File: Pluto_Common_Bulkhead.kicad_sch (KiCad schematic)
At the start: 52 parts

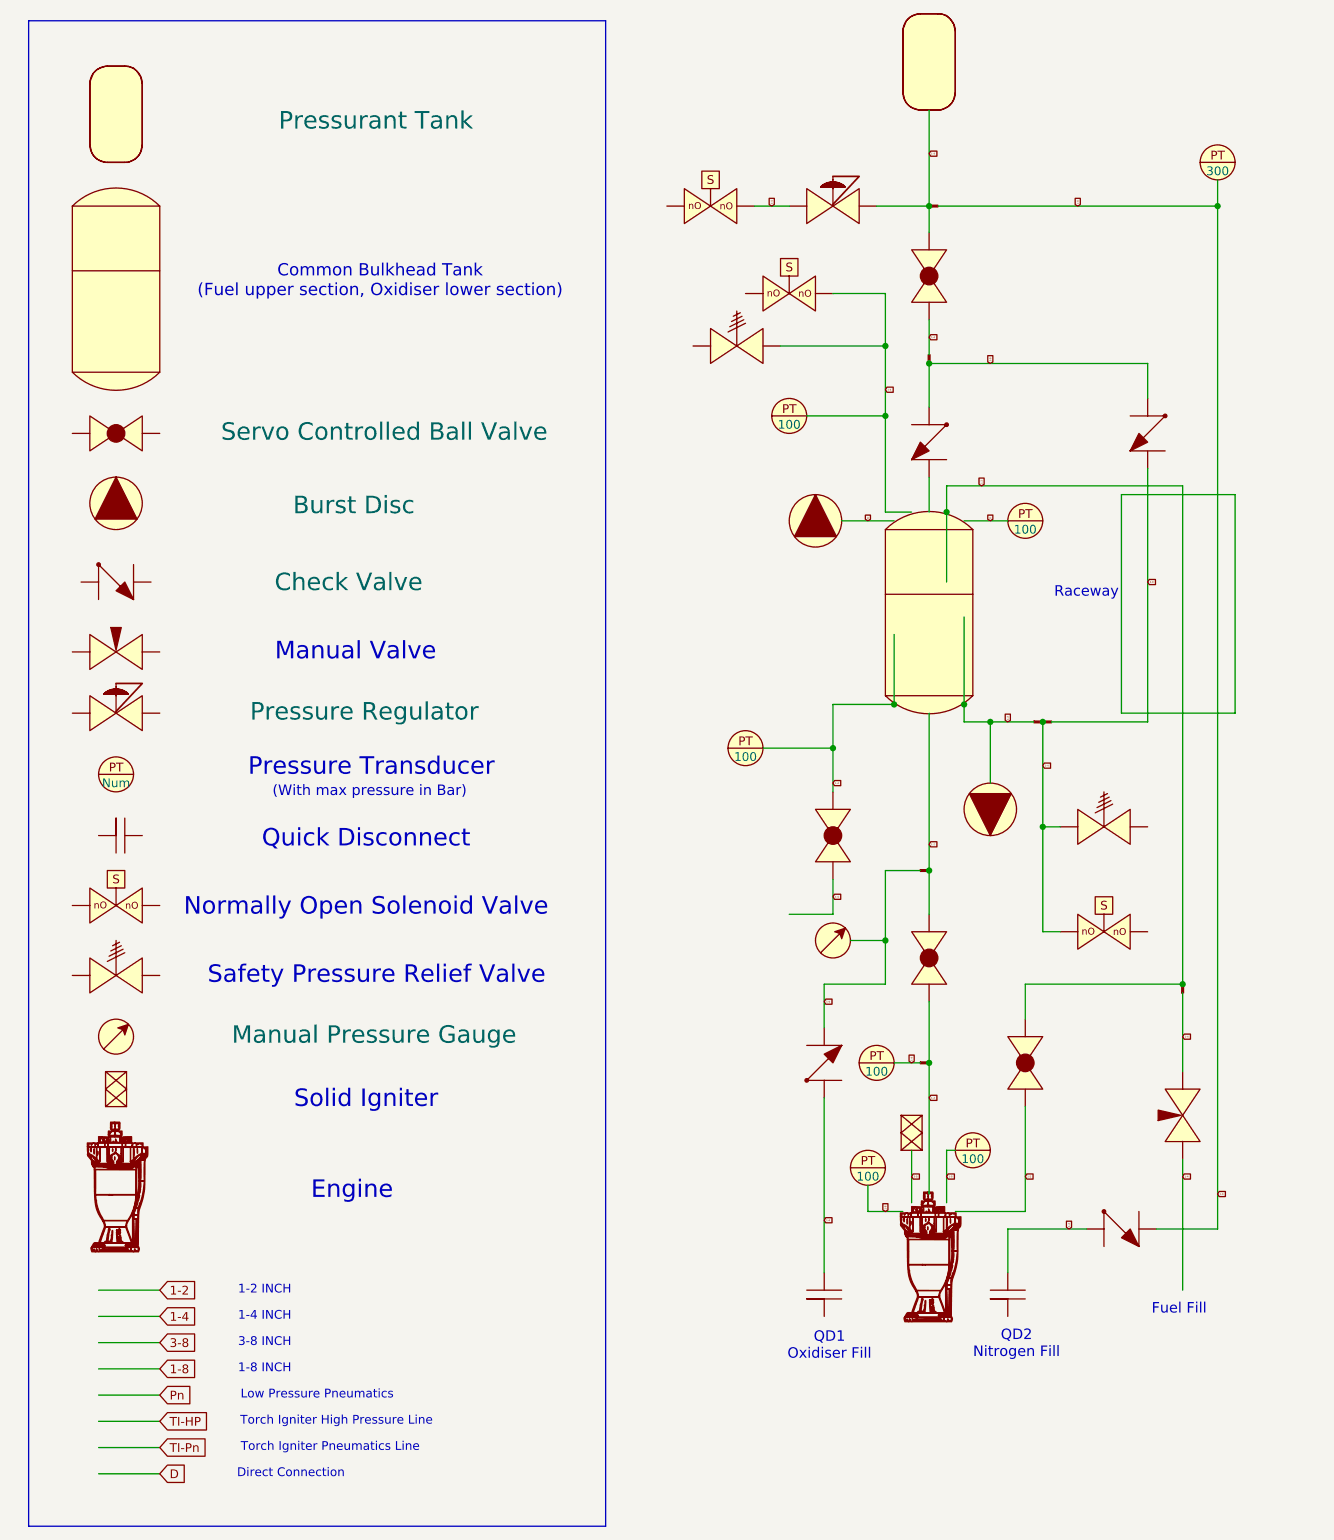
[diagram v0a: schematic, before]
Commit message: more silwood stuff
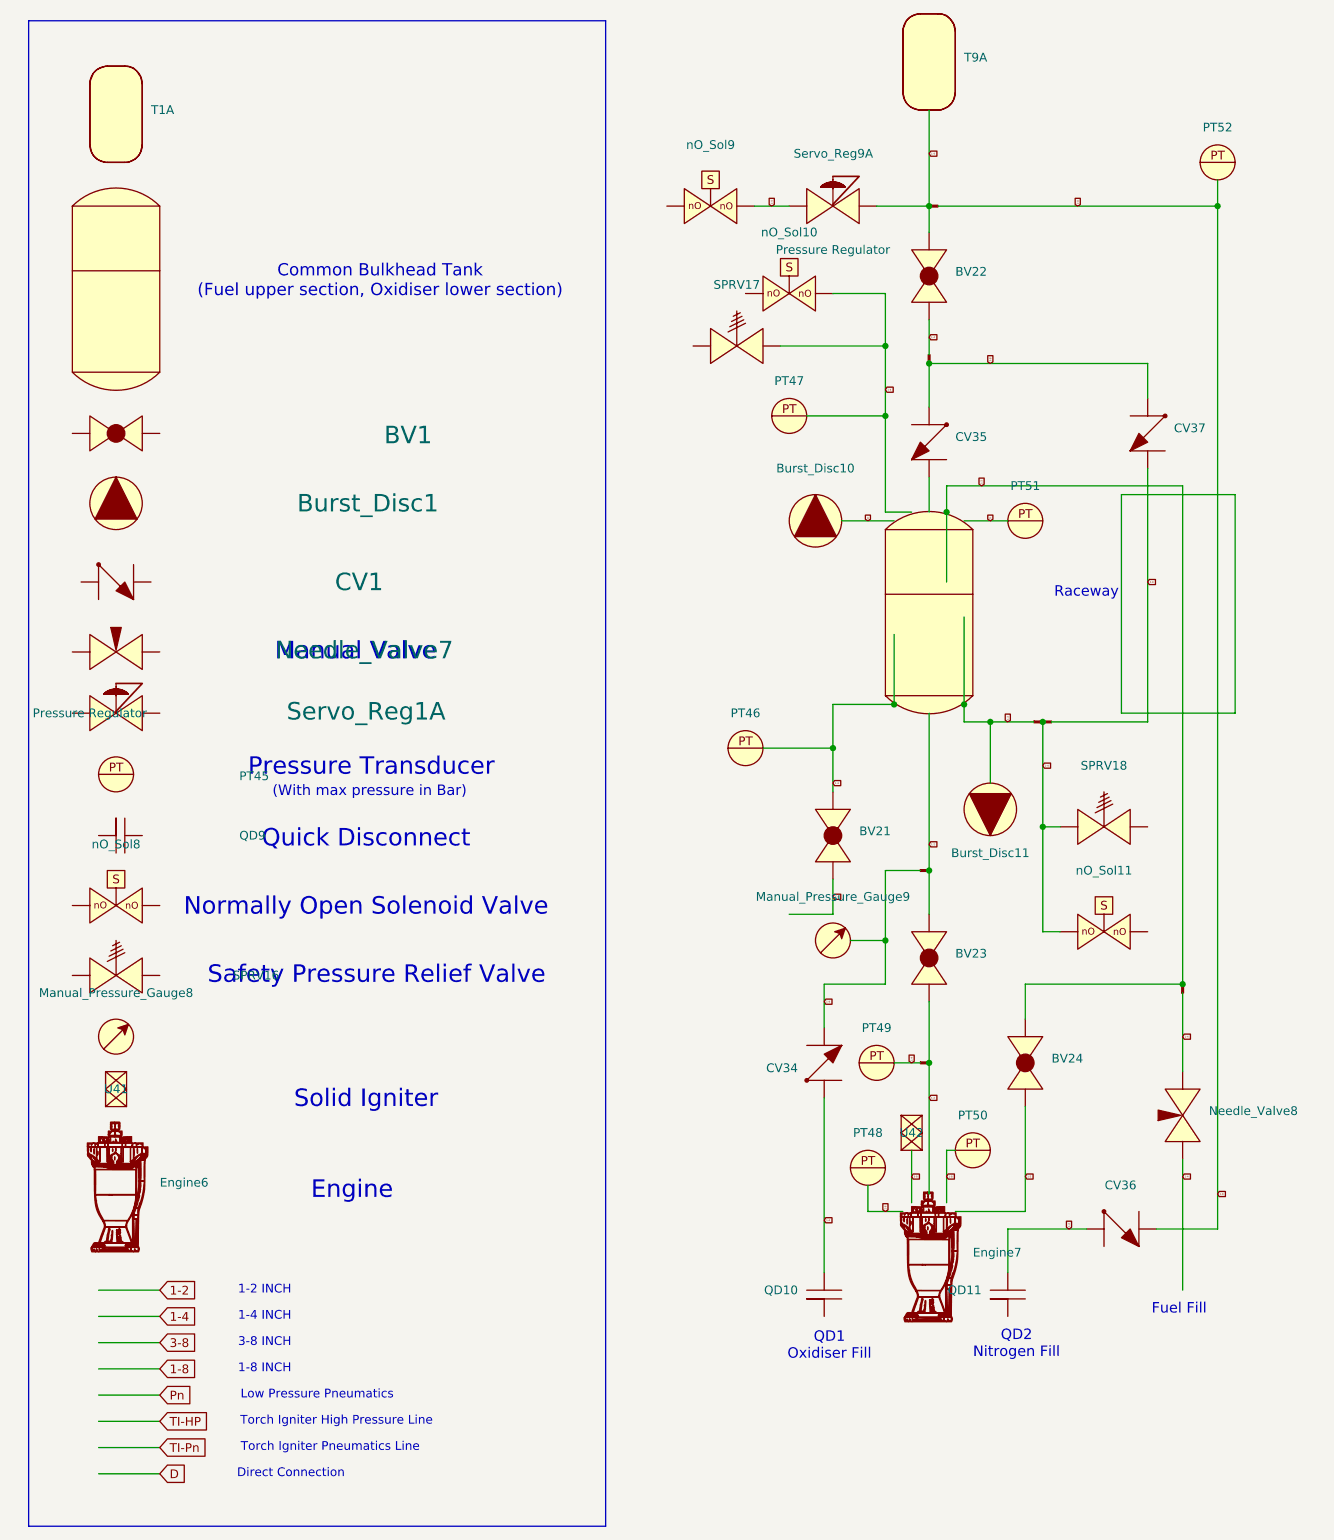
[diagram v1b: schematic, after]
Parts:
- renumbered Ball_Valve(ServoControlled)1 to BV1, BV23 to BV21, BV24 to BV23, BV25 to BV24, BurstDisc1 to Burst_Disc1, Check_Valve1 to CV1, CV36 to CV34, CV37 to CV36, CV34 to CV37, Engine5 to Engine6, Engine6 to Engine7, Manual_Pressure_Gauge7 to Manual_Pressure_Gauge8, Manual_Pressure_Gauge6 to Manual_Pressure_Gauge9, PT36 to PT45, PT35 to PT46, PT33 to PT47, PT39 to PT48, PT37 to PT49, PT38 to PT50, PT34 to PT51, PT32 to PT52, QD9 to QD10, QD10 to QD11, QD8 to QD9, SPRV14 to SPRV17, SPRV15 to SPRV18, Pressure_Regulator1 to Servo_Reg1, Reg9 to Servo_Reg9, Tank1 to T1, U26 to U40, U34 to U41, U35 to U42, U27 to U43, U28 to U44, U31 to U45, U33 to U46, U25 to U47, U29 to U48, U30 to U49, U32 to U50, nO_Sol7 to nO_Sol10, nO_Sol9 to nO_Sol11, nO_Sol6 to nO_Sol9
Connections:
- new net: CV35., U44.

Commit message: Formatiing
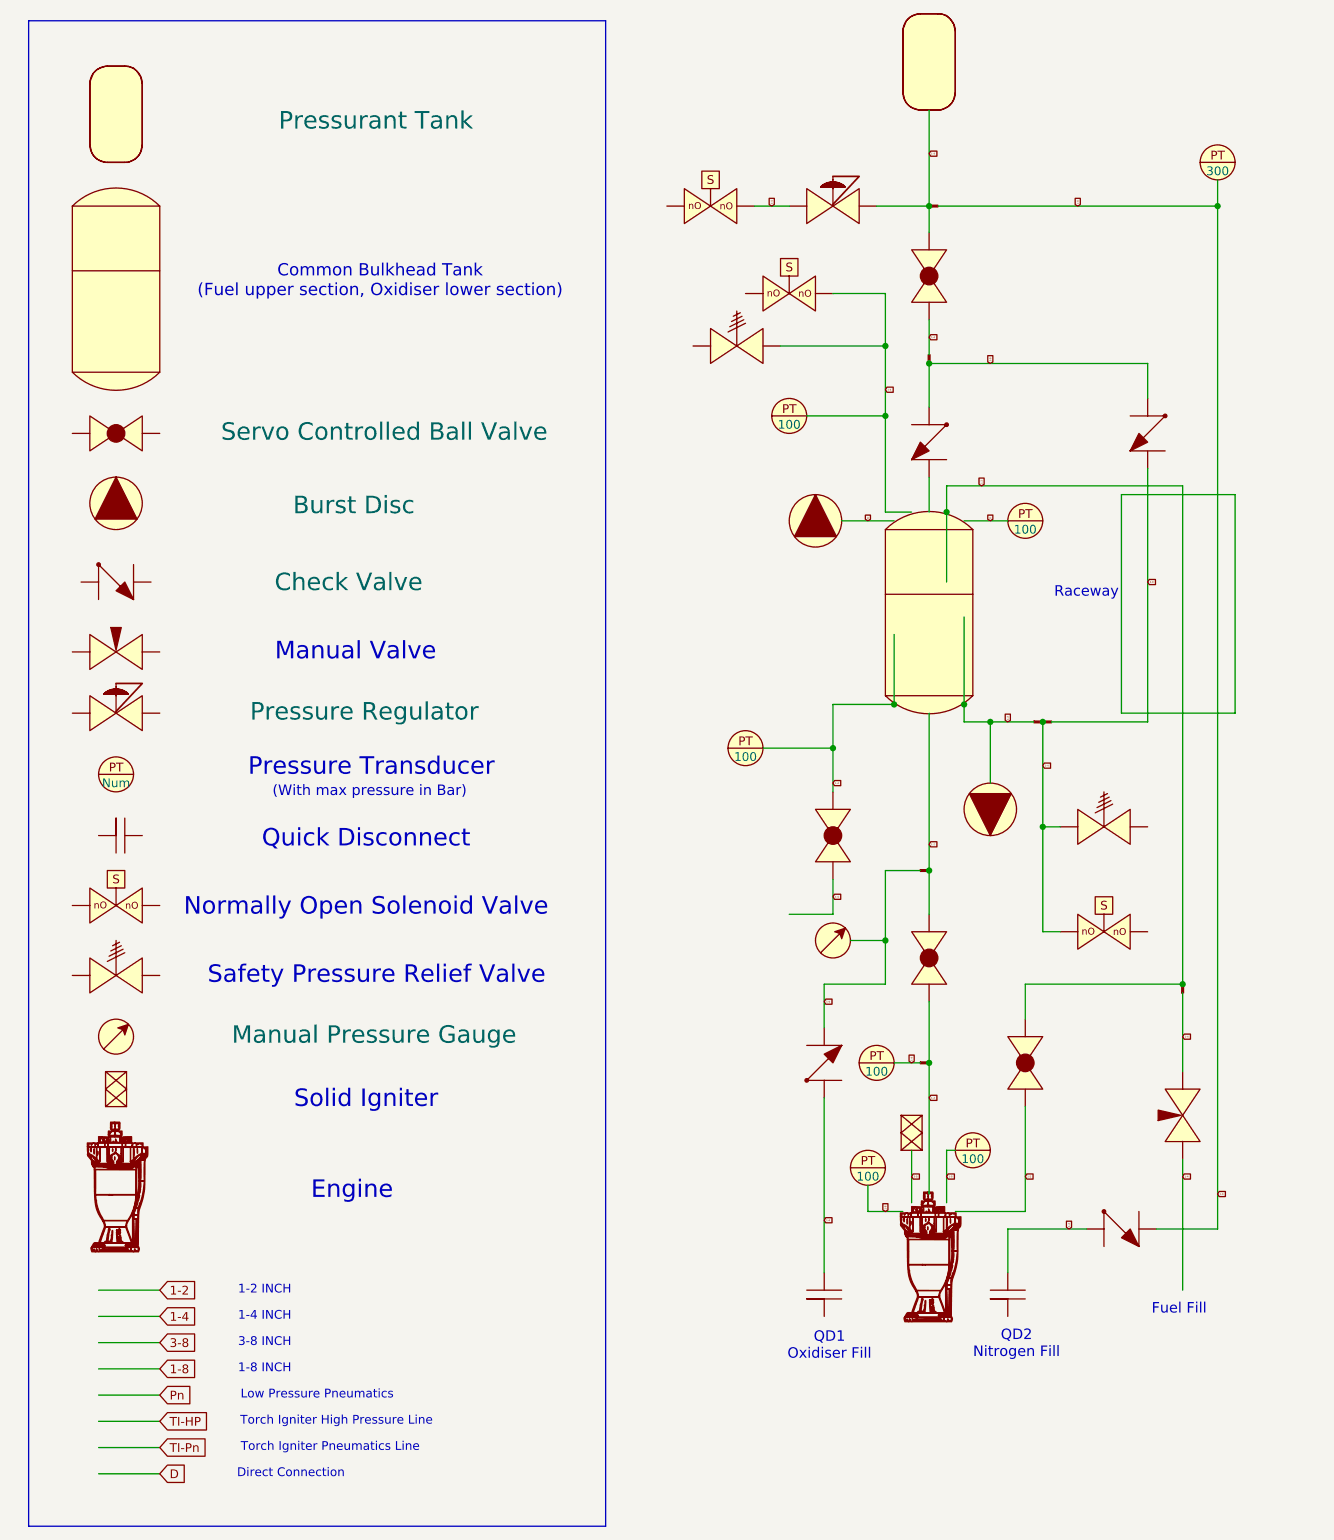
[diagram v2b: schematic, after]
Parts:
- renumbered BV21 to BV53, BV22 to BV54, BV23 to BV55, BV24 to BV56, BV1 to Ball_Valve(ServoControlled)5, Burst_Disc1 to BurstDisc5, Burst_Disc10 to Burst_Disc24, Burst_Disc11 to Burst_Disc25, CV34 to CV55, CV35 to CV56, CV36 to CV57, CV37 to CV58, CV1 to Check_Valve17, Engine6 to Engine18, Engine7 to Engine19, Manual_Pressure_Gauge8 to Manual_Pressure_Gauge11, Manual_Pressure_Gauge9 to Manual_Pressure_Gauge12, Needle_Valve7 to Needle_Valve17, Needle_Valve8 to Needle_Valve18, PT51 to PT100, PT52 to PT101, PT45 to PT94, PT46 to PT95, PT47 to PT96, PT48 to PT97, PT49 to PT98, PT50 to PT99, Servo_Reg1 to Pressure_Regulator5, QD9 to QD38, QD10 to QD39, QD11 to QD40, Servo_Reg9 to Reg23, SPRV16 to SPRV32, SPRV17 to SPRV33, SPRV18 to SPRV34, T9 to T17, T1 to Tank5, U40 to U53, U41 to U54, U42 to U55, U43 to U56, U44 to U57, U45 to U58, U46 to U59, U47 to U60, U48 to U61, U49 to U62, U50 to U63, nO_Sol8 to nO_Sol34, nO_Sol9 to nO_Sol35, nO_Sol10 to nO_Sol36, nO_Sol11 to nO_Sol37
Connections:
- new net: CV56., U57.
